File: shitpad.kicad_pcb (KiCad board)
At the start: 2 copper layers, 33 x 68 mm, 20 parts, among them J1 Shitty Connector, J2 Conn_01x04, J3 Conn_01x09, J4 Conn_02x05_Top_Bottom

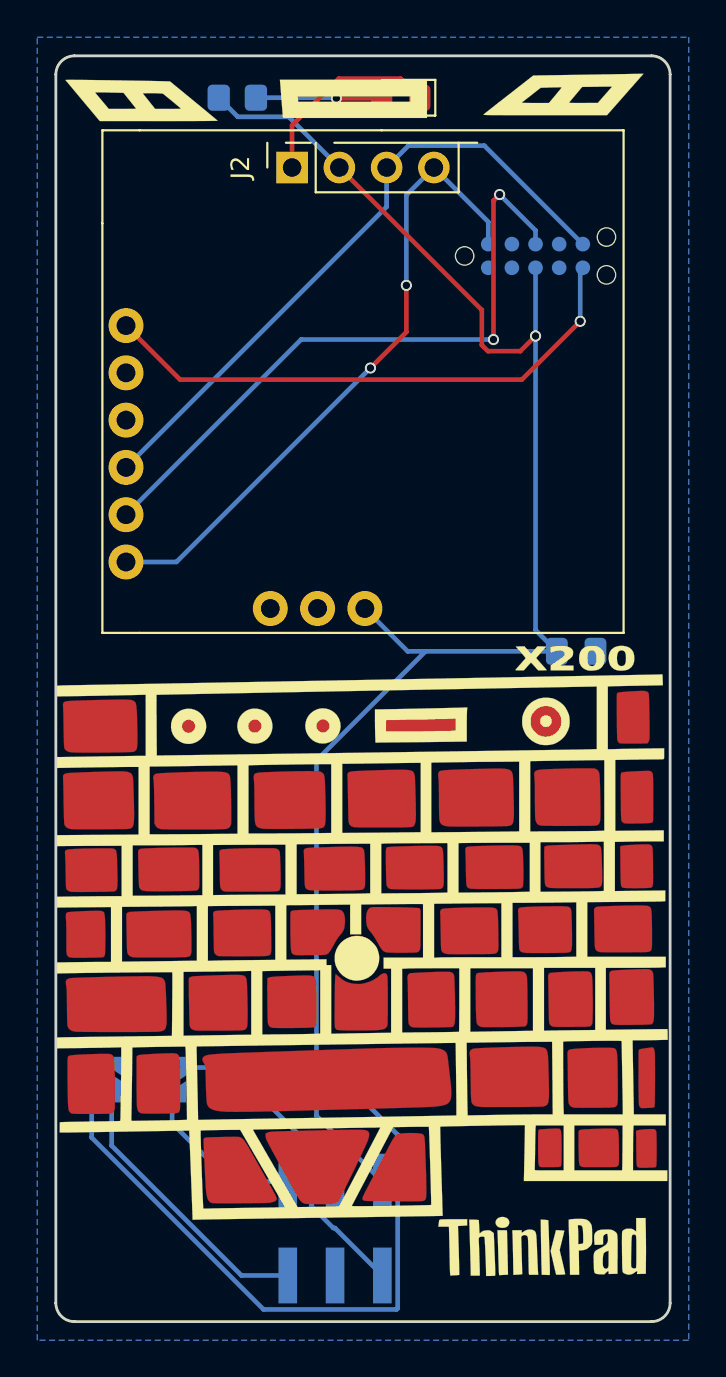
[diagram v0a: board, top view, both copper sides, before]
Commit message: round 2
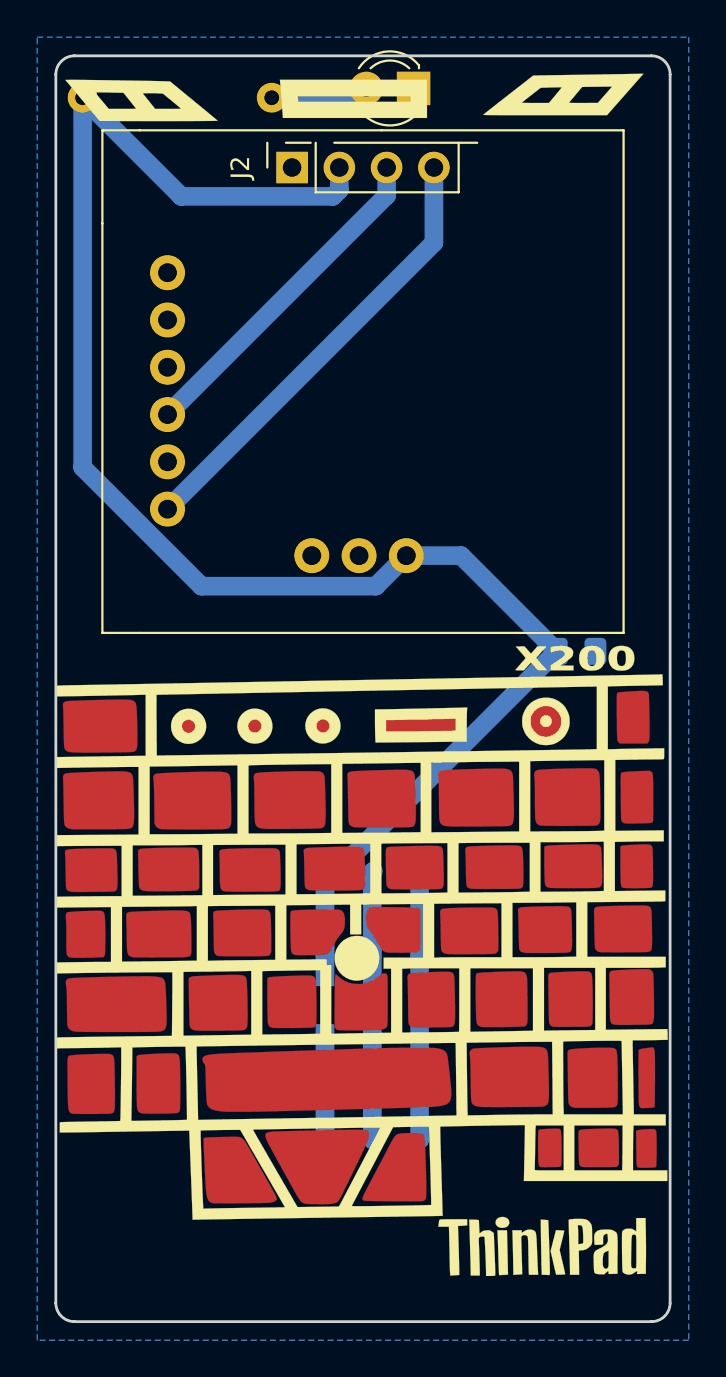
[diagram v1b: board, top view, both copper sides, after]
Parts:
- removed the G*** at (0.00, 0.00) (x5)
- removed J4: Conn_02x05_Top_Bottom, Connector:Tag-Connect_TC2050-IDC-NL_2x05_P1.27mm_Vertical
- removed JP1: VJ, Jumper:SolderJumper-2_P1.3mm_Bridged_RoundedPad1.0x1.5mm
- removed JP2: ~GJ, Jumper:SolderJumper-2_P1.3mm_Open_TrianglePad1.0x1.5mm
- removed JP3: GJ, Jumper:SolderJumper-2_P1.3mm_Bridged_RoundedPad1.0x1.5mm
- removed JP4: ~VJ, Jumper:SolderJumper-2_P1.3mm_Open_TrianglePad1.0x1.5mm
- added G***: LOGO, shitpad:lenowo, B.Cu at (84.4, 93.2)
- added G*** (x5): LOGO, LOGO, F.Cu at (0.00, 0.00)
- C1: value C_Small -> 100nF
- D1: footprint LED_SMD:LED_0805_2012Metric_Pad1.15x1.40mm_HandSolder -> LED_THT:LED_D3.0mm
- R1: footprint Resistor_SMD:R_0805_2012Metric_Pad1.20x1.40mm_HandSolder -> Resistor_THT:R_Axial_DIN0207_L6.3mm_D2.5mm_P10.16mm_Horizontal
- moved G*** 21.7 mm to (101.4, 35.6)
- moved J1 12.2 mm to (91.0, 81.0)
- moved R1 8.31 mm to (75.4, 32.2)
- moved G*** 5.81 mm to (84.3, 67.8)
- moved J3 3.61 mm to (80.0, 48.0)
- moved D1 0.85 mm to (93.2, 31.8)
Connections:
- J1 pad 5: Net-(J1-Pad5) -> +3V3
- J1 pad 6: Net-(J1-Pad6) -> GND
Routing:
- net /CIPO: track 35.0 -> 0.00 mm, vias 2 -> 0
- net +3V3: track 121.4 -> 89.8 mm, vias 1 -> 0
- net /NRST: track 29.8 -> 0.00 mm, vias 1 -> 0
- net /SCL: track 35.1 -> 18.1 mm
- net Net-(J1-Pad6): track 15.2 -> 0.00 mm
- net /SDA: track 35.0 -> 24.3 mm, vias 2 -> 0
- net GND: track 14.4 -> 4.84 mm
- net Net-(J1-Pad5): track 9.13 -> 0.00 mm
- net Net-(J1-Pad2): track 13.5 -> 4.72 mm
- net Net-(J1-Pad4): track 0.00 -> 4.72 mm
- net Net-(J1-Pad3): track 0.00 -> 4.71 mm
- net Net-(D1-Pad2): track 6.77 -> 5.29 mm, vias 1 -> 0
- net Net-(J1-Pad1): track 6.30 -> 5.15 mm
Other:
- net class Default removed
- board text added: "I bet your bios is stock baka~"
- board text removed: "I bet your bios is stock~ baka~"
- board text removed: "in case of fuck up cut JP1 and JP3 bridge JP2 and JP4"
